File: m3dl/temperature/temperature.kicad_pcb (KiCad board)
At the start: 2 copper layers, 40 x 33 mm, 44 parts, among them IC1 LTC2983, J1 WEST TOP, J2 EAST TOP, J3 WEST BOT, J4 EAST BOT, J5 SOUTH TOP, J6 SOUTH BOT, J7 TEMP1, J8 TEMP9, J9 TEMP2-8

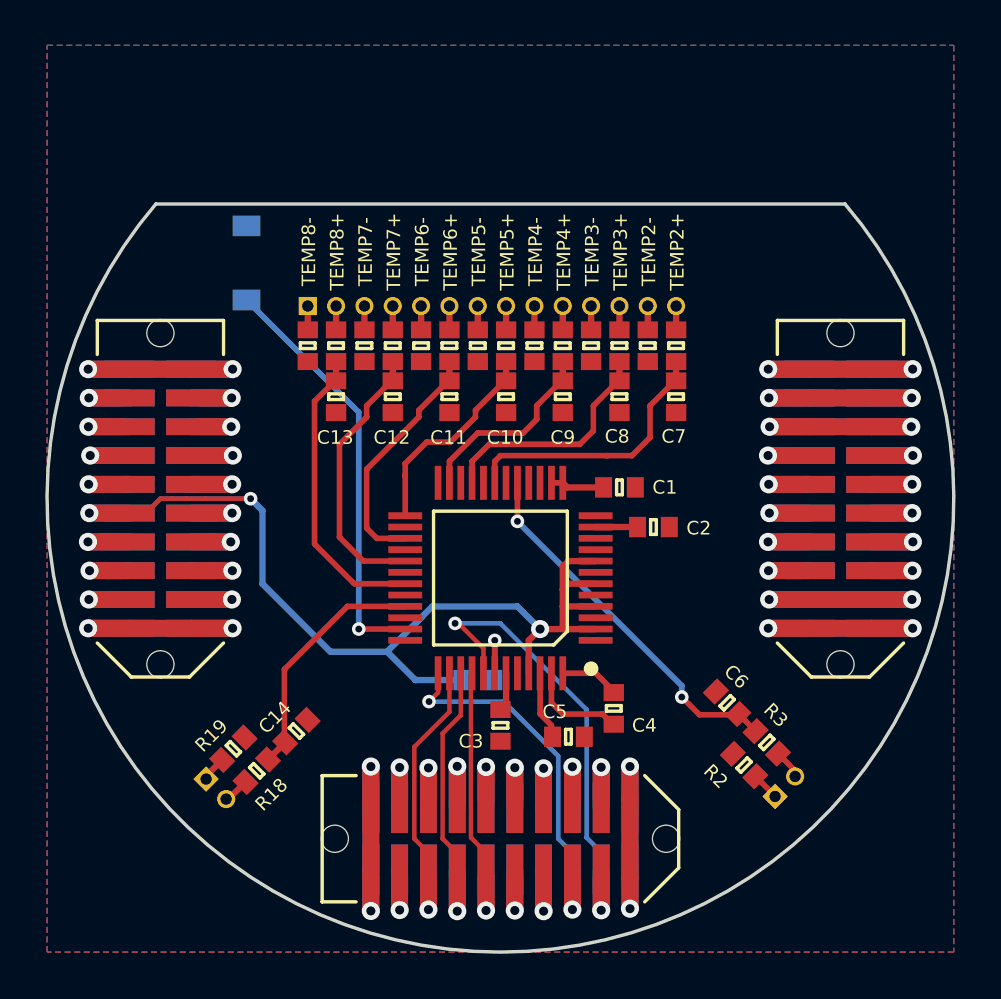
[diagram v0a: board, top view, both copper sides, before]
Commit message: Almost ready to generate gerbers
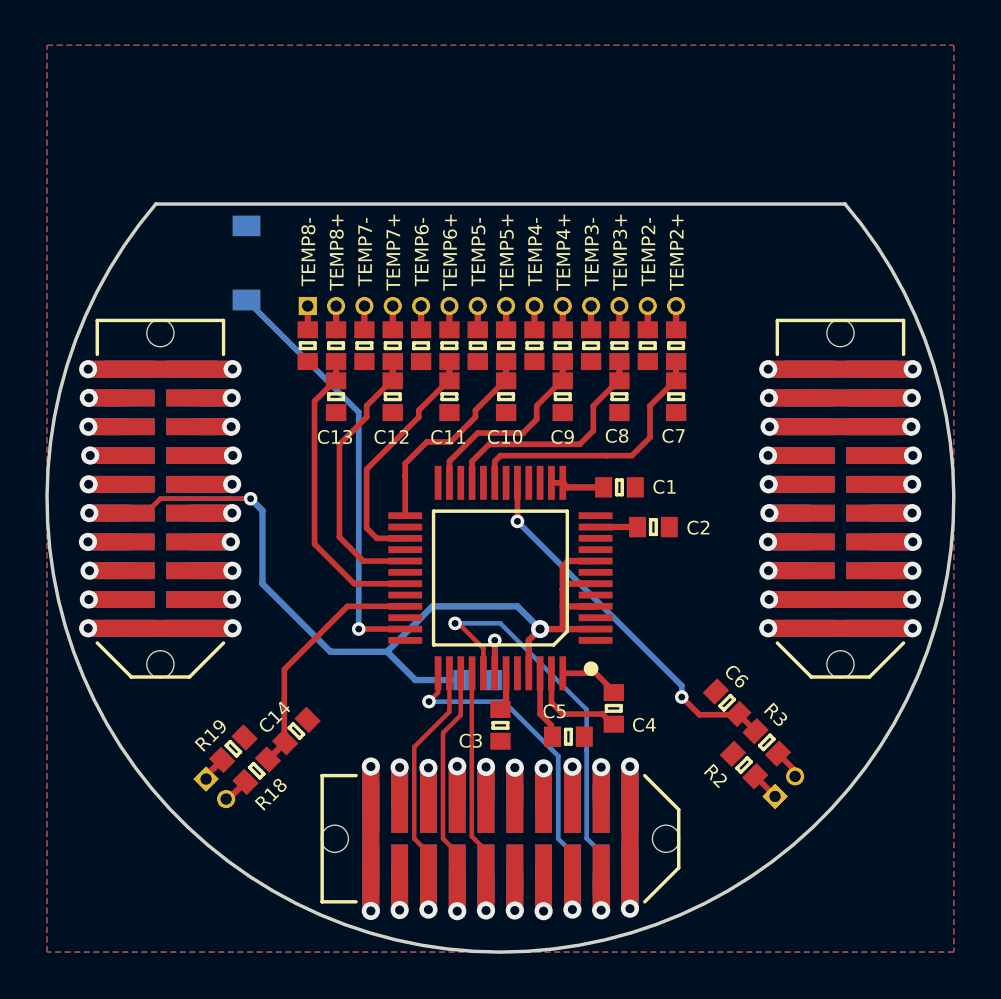
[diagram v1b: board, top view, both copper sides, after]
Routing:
- net /SPI1_MOSI: track 12.6 -> 13.7 mm
- net /SPI1_MISO: track 12.9 -> 14.0 mm
- net /SPI1_CS: track 20.7 -> 21.5 mm
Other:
- net class Default: clearance 0.1 -> 0.127
- rule pad_to_mask_clearance: 0.2 -> 0
- rule trace_clearance: 0.1 -> 0.127
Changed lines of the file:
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@@
     (thickness 1.6)
     (drawings 60)
-    (tracks 378)
+    (tracks 385)
     (zones 0)
     (modules 44)
@@
     (user_trace_width 0.28)
     (user_trace_width 0.74)
-    (trace_clearance 0.1)
+    (trace_clearance 0.127)
     (zone_clearance 0.15)
     (zone_45_only no)
@@
     (pad_size 1.524 1.524)
     (pad_drill 0.762)
-    (pad_to_mask_clearance 0.2)
+    (pad_to_mask_clearance 0)
     (aux_axis_origin 0 0)
     (visible_elements FFFFFE1F)
@@
   (net 83 /TEMP9-)
   (net_class Default "This is the default net class."
-    (clearance 0.1)
+    (clearance 0.127)
     (trace_width 0.25)
     (via_dia 0.6)
@@
     (effects (font (size 0.6 0.6) (thickness 0.12)))
   )
-  (gr_text C1 (at 107.25 99.5 360) (layer F.SilkS)
+  (gr_text C1 (at 107.25 99.5) (layer F.SilkS)
     (effects (font (size 0.6 0.6) (thickness 0.12)))
   )
@@
   (segment (start 93.75 96.185) (end 93.75 105.75) (width 0.25) (layer B.Cu) (net 16))
   (segment (start 88.8 91.235) (end 93.75 96.185) (width 0.25) (layer B.Cu) (net 16))
+  (segment (start 103.175 116.365) (end 103.175 115.625) (width 0.2) (layer B.Cu) (net 17))
+  (segment (start 103.175 115.625) (end 102.547999 114.997999) (width 0.2) (layer B.Cu) (net 17))
+  (segment (start 102.547999 114.997999) (end 102.547999 111.352001) (width 0.2) (layer B.Cu) (net 17))
+  (segment (start 102.547999 111.352001) (end 102.55 111.35) (width 0.2) (layer B.Cu) (net 17))
   (segment (start 96.85 108.95) (end 100.15 108.95) (width 0.2) (layer B.Cu) (net 17))
   (segment (start 100.15 108.95) (end 102.55 111.35) (width 0.2) (layer B.Cu) (net 17))
@@
   (segment (start 97.25 108.55) (end 96.85 108.95) (width 0.2) (layer F.Cu) (net 17))
   (segment (start 97.25 107.7) (end 97.25 108.55) (width 0.2) (layer F.Cu) (net 17))
-  (segment (start 102.55 115) (end 102.55 111.35) (width 0.2) (layer B.Cu) (net 17))
-  (segment (start 103.175 115.625) (end 102.55 115) (width 0.2) (layer B.Cu) (net 17))
-  (segment (start 103.175 116.365) (end 103.175 115.625) (width 0.2) (layer B.Cu) (net 17))
   (segment (start 103.175 116.365) (end 103.175 118.125) (width 0.74) (layer B.Cu) (net 17))
   (via (at 103.175 118.125) (size 0.8) (drill 0.4) (layers F.Cu B.Cu) (net 17))
   (segment (start 103.175 116.715) (end 103.175 118.125) (width 0.74) (layer F.Cu) (net 17))
-  (segment (start 96.2 115) (end 96.825 115.625) (width 0.2) (layer F.Cu) (net 18))
-  (segment (start 96.825 115.625) (end 96.825 116.715) (width 0.2) (layer F.Cu) (net 18))
-  (segment (start 96.2 110.95) (end 96.2 115) (width 0.2) (layer F.Cu) (net 18))
-  (segment (start 97.75 109.4) (end 96.2 110.95) (width 0.2) (layer F.Cu) (net 18))
-  (segment (start 97.75 107.7) (end 97.75 109.4) (width 0.2) (layer F.Cu) (net 18))
+  (segment (start 96.825 116.715) (end 96.825 115.625) (width 0.2) (layer F.Cu) (net 18))
+  (segment (start 96.825 115.625) (end 96.197999 114.997999) (width 0.2) (layer F.Cu) (net 18))
+  (segment (start 96.197999 114.997999) (end 96.197999 110.952001) (width 0.2) (layer F.Cu) (net 18))
+  (segment (start 96.197999 110.952001) (end 97.75 109.4) (width 0.2) (layer F.Cu) (net 18))
+  (segment (start 97.75 109.4) (end 97.75 107.7) (width 0.2) (layer F.Cu) (net 18))
   (segment (start 96.825 116.365) (end 96.825 118.125) (width 0.74) (layer B.Cu) (net 18))
   (via (at 96.825 118.125) (size 0.8) (drill 0.4) (layers F.Cu B.Cu) (net 18))
   (segment (start 96.825 116.715) (end 96.825 118.125) (width 0.74) (layer F.Cu) (net 18))
-  (segment (start 98.25 107.7) (end 98.25 109.55) (width 0.2) (layer F.Cu) (net 19))
-  (segment (start 98.25 109.55) (end 97.45 110.35) (width 0.2) (layer F.Cu) (net 19))
-  (segment (start 97.45 110.35) (end 97.45 115) (width 0.2) (layer F.Cu) (net 19))
-  (segment (start 97.45 115) (end 98.095 115.645) (width 0.2) (layer F.Cu) (net 19))
+  (segment (start 98.095 116.715) (end 98.095 115.625) (width 0.2) (layer F.Cu) (net 19))
+  (segment (start 98.095 115.625) (end 97.467999 114.997999) (width 0.2) (layer F.Cu) (net 19))
+  (segment (start 97.467999 110.332001) (end 98.25 109.55) (width 0.2) (layer F.Cu) (net 19))
+  (segment (start 97.467999 114.997999) (end 97.467999 110.332001) (width 0.2) (layer F.Cu) (net 19))
+  (segment (start 98.25 109.55) (end 98.25 107.7) (width 0.2) (layer F.Cu) (net 19))
   (segment (start 98.095 115.645) (end 98.095 116.715) (width 0.2) (layer F.Cu) (net 19))
   (segment (start 98.095 116.365) (end 98.095 118.195) (width 0.74) (layer B.Cu) (net 19))
   (via (at 98.095 118.195) (size 0.8) (drill 0.4) (layers F.Cu B.Cu) (net 19))
   (segment (start 98.095 116.715) (end 98.095 118.195) (width 0.74) (layer F.Cu) (net 19))
+  (segment (start 99.365 116.715) (end 99.365 115.523602) (width 0.2) (layer F.Cu) (net 20))
+  (segment (start 98.737999 114.896601) (end 98.737999 107.712001) (width 0.2) (layer F.Cu) (net 20))
+  (segment (start 99.365 115.523602) (end 98.737999 114.896601) (width 0.2) (layer F.Cu) (net 20))
+  (segment (start 98.737999 107.712001) (end 98.75 107.7) (width 0.2) (layer F.Cu) (net 20))
   (segment (start 99.365 116.715) (end 99.365 115.615) (width 0.2) (layer F.Cu) (net 20))
-  (segment (start 99.365 115.615) (end 98.7 114.95) (width 0.2) (layer F.Cu) (net 20))
-  (segment (start 98.7 114.95) (end 98.7 107.75) (width 0.2) (layer F.Cu) (net 20))
   (segment (start 98.7 107.75) (end 98.75 107.7) (width 0.2) (layer F.Cu) (net 20))
   (segment (start 99.365 116.365) (end 99.365 118.165) (width 0.74) (layer B.Cu) (net 20))
   (via (at 99.365 118.165) (size 0.8) (drill 0.4) (layers F.Cu B.Cu) (net 20))
   (segment (start 99.365 116.715) (end 99.365 118.165) (width 0.74) (layer F.Cu) (net 20))
+  (segment (start 103.802001 111.102001) (end 103.8 111.1) (width 0.2) (layer B.Cu) (net 21))
+  (segment (start 103.8 111.1) (end 103.8 109.3) (width 0.2) (layer B.Cu) (net 21))
+  (segment (start 104.445 116.365) (end 104.445 115.625) (width 0.2) (layer B.Cu) (net 21))
+  (segment (start 104.445 115.625) (end 103.802001 114.982001) (width 0.2) (layer B.Cu) (net 21))
+  (segment (start 103.802001 114.982001) (end 103.802001 111.102001) (width 0.2) (layer B.Cu) (net 21))
   (segment (start 98 105.5) (end 98.15 105.5) (width 0.2) (layer F.Cu) (net 21))
   (segment (start 98.15 105.5) (end 99.25 106.6) (width 0.2) (layer F.Cu) (net 21))
@@
   (segment (start 98 105.5) (end 100 105.5) (width 0.2) (layer B.Cu) (net 21))
   (segment (start 100 105.5) (end 103.8 109.3) (width 0.2) (layer B.Cu) (net 21))
-  (segment (start 103.8 114.95) (end 104.445 115.595) (width 0.2) (layer B.Cu) (net 21))
-  (segment (start 103.8 109.3) (end 103.8 114.95) (width 0.2) (layer B.Cu) (net 21))
   (segment (start 104.445 115.595) (end 104.445 116.365) (width 0.2) (layer B.Cu) (net 21))
   (via (at 98 105.5) (size 0.6) (drill 0.3) (layers F.Cu B.Cu) (net 21))
